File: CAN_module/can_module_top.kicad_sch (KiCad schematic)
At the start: 56 parts, among them IC1 SN65HVD233QDRQ1, J2 Barrel_Jack_Switch, J4 Conn_Coaxial, J5 Screw_Terminal_01x02, U1 PC817, U2 LM5164QDDATQ1, U3 Antena BT - 2450AT42E010B001E

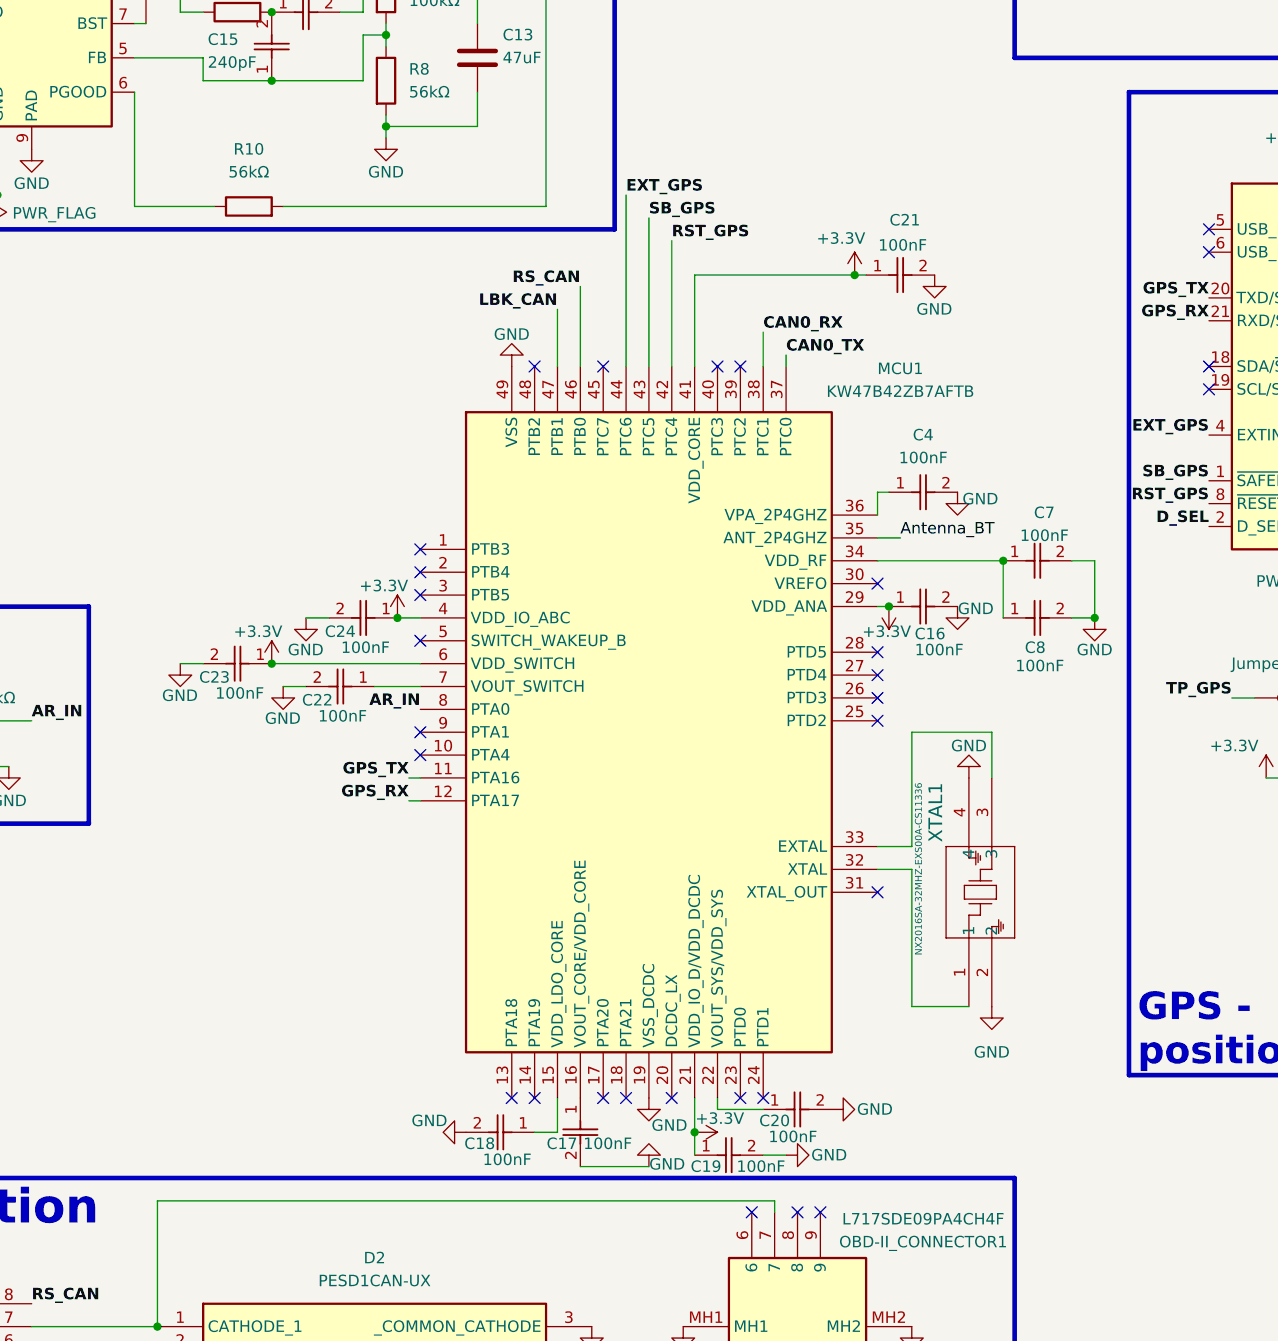
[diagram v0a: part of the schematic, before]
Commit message: Add files via upload
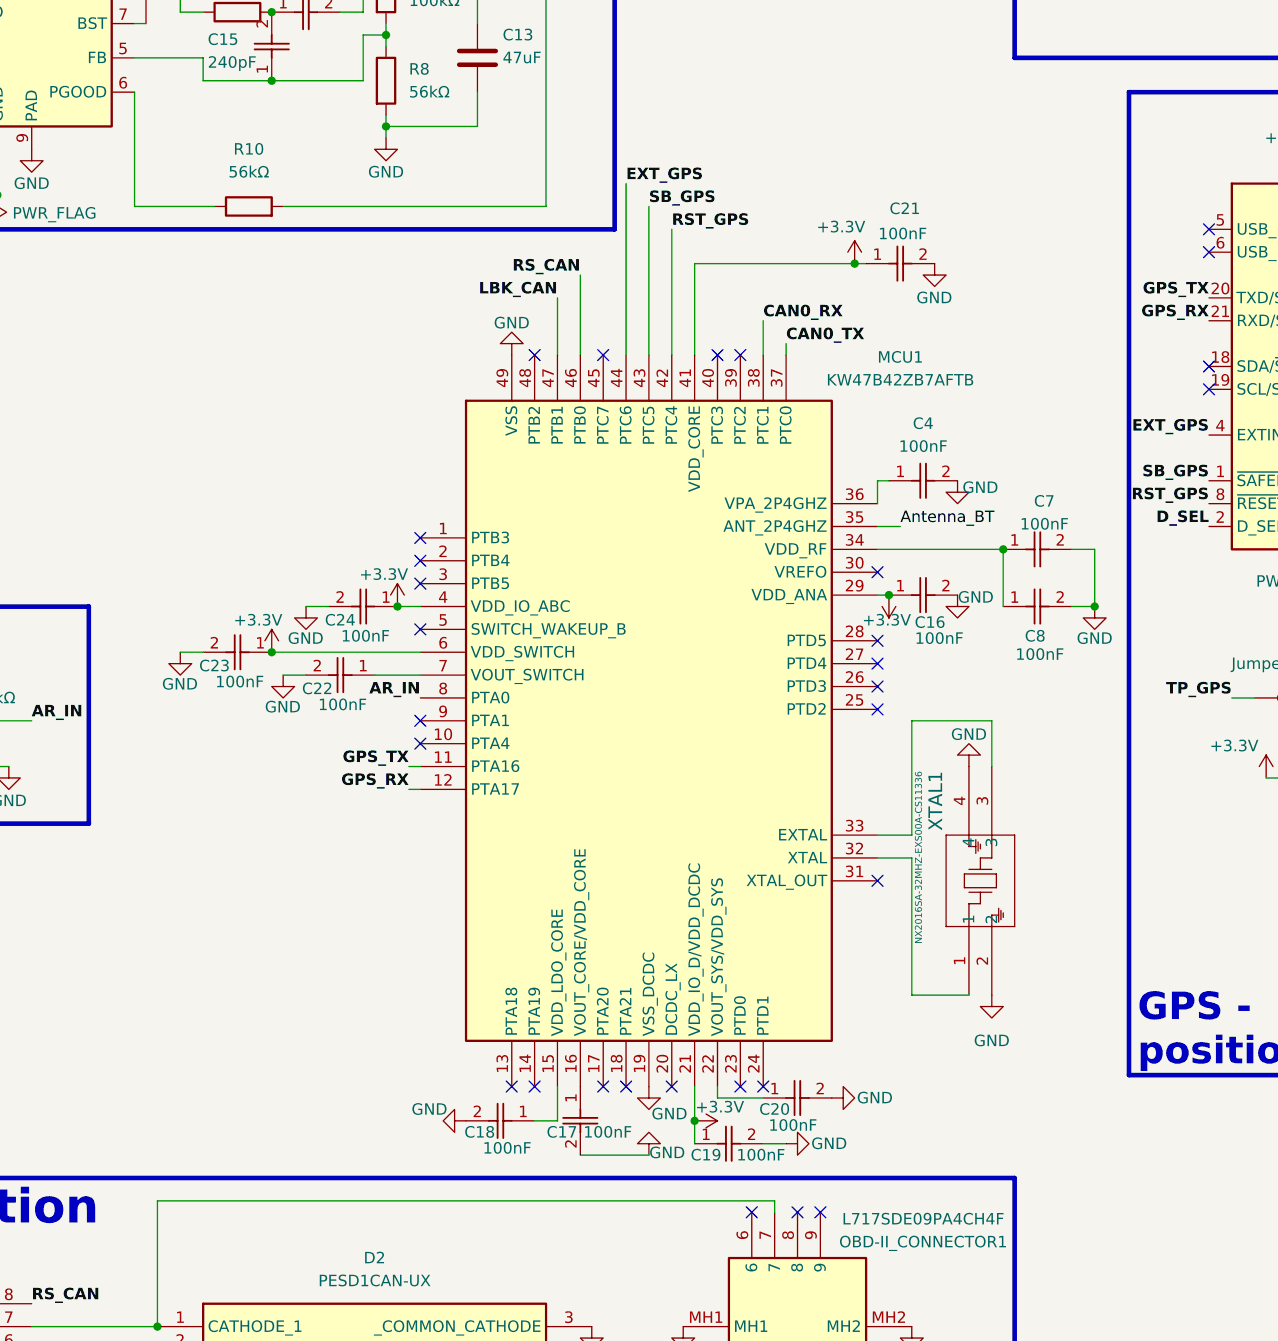
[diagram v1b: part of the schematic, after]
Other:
- company: (none) -> Tobiasz Kobza; Mikołaj Krok; Adam Michalik
- title: (none) -> Schemat elektroniczny modułu PCB antyradar-CAN
- moved on the sheet: C16, C17, C18, C19, C20, C21, C22, C23, C24, C4, C7, C8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
